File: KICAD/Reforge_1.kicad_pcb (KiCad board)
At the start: 2 copper layers, 57.9 x 76 mm, 94 parts, among them J1 USB_C_Receptacle_USB2.0_16P, J10 Conn_01x14_Pin, J11 Conn_01x12_Pin, J12 Conn_01x12_Pin, J14 Conn_01x12_Pin, J15 Conn_01x12_Pin, J3 Conn_01x02, J8 Conn_01x12_Pin, J9 Conn_01x14_Pin, Q1 SS8050, Q2 SS8050, SW1 SW_Push, SW2 SW_Push, U11 SN74LVC2G125DCUR, U2 CP2102N-Axx-xQFN28, U3 ICE40UP5K-SG48ITR, U4 AP2112K-1.2, U5 ESP32-WROOM-32D, U6 AMS1117-3.3, U8 W25Q32JVSS, Y1 SG-210STF

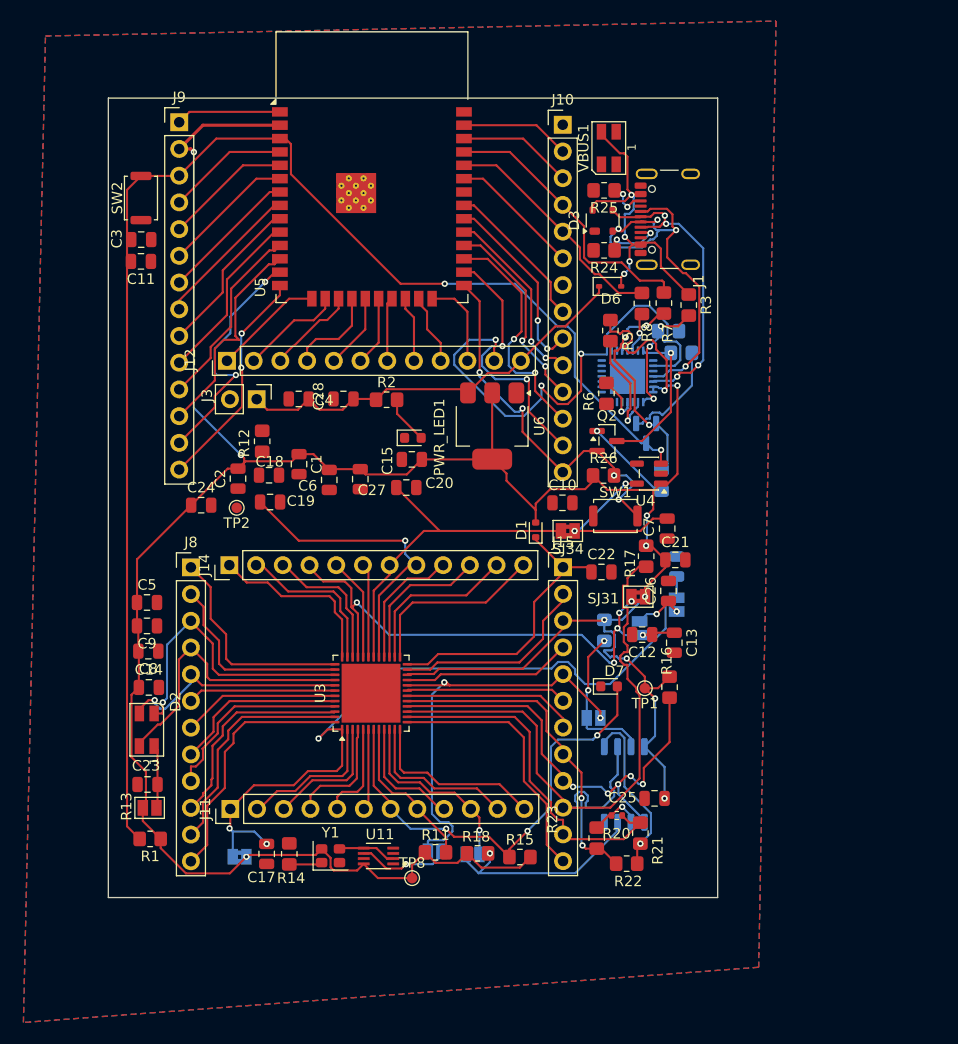
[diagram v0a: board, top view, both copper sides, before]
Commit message: Update schematic and PCB
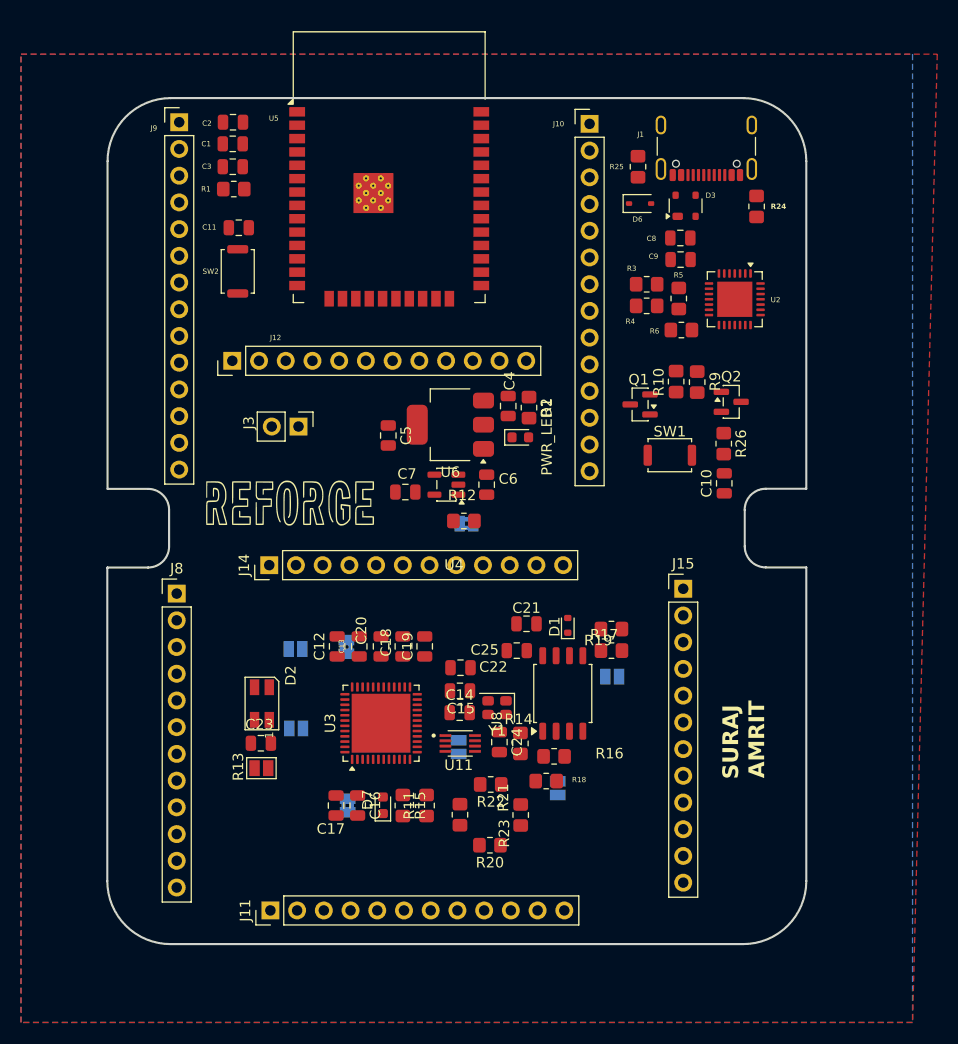
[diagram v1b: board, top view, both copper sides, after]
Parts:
- removed C26, C27, C28: DNI, Capacitor_SMD:C_0805_2012Metric
- removed the G*** at (130.1, 58.2)
- removed R7, R8: 0R(5%), Resistor_SMD:R_0805_2012Metric_Pad1.20x1.40mm_HandSolder
- removed TP1, TP2, TP8: TestPoint, TestPoint:TestPoint_Pad_D1.0mm
- removed VBUS1: TestPoint, LED_SMD:LED_RGB_Wuerth-PLCC4_3.2x2.8mm_150141M173100
- added G***: LOGO, LOGO, F.Cu at (122.5, 87.4)
- added G***: LOGO, LOGO, B.Cu at (129.5, 60.2)
- added G***: LOGO, LOGO, B.Cu at (158.5, 66.4)
- C16, Q1, R10, R19, R4, R9, U2, U8: moved to F.Cu
- R20: footprint Resistor_SMD:R_0402_1005Metric -> Resistor_SMD:R_0805_2012Metric_Pad1.20x1.40mm_HandSolder
- SJ31, SJ34: moved to B.Cu
- moved C8 64.0 mm to (159.4, 60.4), turned to 0 degrees
- moved R1 62.3 mm to (117.0, 55.8)
- moved C9 61.5 mm to (159.4, 62.5), turned to 0 degrees
- moved SJ26 38.0 mm to (122.9, 107.0), turned to 0 degrees
- moved C16 37.9 mm to (128.7, 114.4), turned to -90 degrees
- moved C24 36.2 mm to (142.2, 108.3), turned to -90 degrees
- moved C2 33.9 mm to (116.9, 49.4), turned to 0 degrees
- moved SJ19 32.8 mm to (122.8, 99.5), turned to 0 degrees
- moved C1 31.1 mm to (116.8, 51.5), turned to 180 degrees
- moved C13 30.0 mm to (128.9, 99.2), turned to 90 degrees
- moved C14 29.6 mm to (138.4, 105.5)
- moved C12 29.0 mm to (126.8, 99.2), turned to 90 degrees
- moved SJ31 28.2 mm to (127.7, 99.3), turned to -90 degrees
- moved C5 27.9 mm to (131.6, 79.2), turned to -90 degrees
- moved C7 25.1 mm to (133.3, 84.6), turned to 180 degrees
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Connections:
- J10 pad 4: /TXD0 -> /RXD
- Q2 pad 2: /IO0 -> /~{DTR}
- Q2 pad 3: /~{DTR} -> /IO0
- U2 pad 26: /TXD -> /RXD0
- U5 pad 35: /TXD0 -> /RXD
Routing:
- net /VDD33: track 275.1 -> 0.00 mm, vias 12 -> 0
- net /EN: track 132.6 -> 0.00 mm, vias 2 -> 0
- net /VCCIO_2: track 72.4 -> 0.00 mm, vias 3 -> 0
- net /FT_SCK: track 67.6 -> 0.00 mm
- net /VCCIO_0: track 51.8 -> 0.00 mm, vias 6 -> 0
- net /CLK: track 48.1 -> 0.00 mm, vias 3 -> 0
- net /CDONE: track 43.8 -> 0.00 mm, vias 3 -> 0
- net /FT_SSn: track 43.0 -> 0.00 mm, vias 5 -> 0
- net /+1.2V_CORE: track 42.3 -> 0.00 mm
- net /USB_DP: track 41.2 -> 0.00 mm, vias 4 -> 0
- net /IOB_25B_G3: track 41.1 -> 0.00 mm, vias 2 -> 0
- net /EXT_5V: track 39.4 -> 0.00 mm
- net /IO0: track 36.2 -> 0.00 mm, vias 4 -> 0
- net /FPGA_SO: track 33.8 -> 0.00 mm
- net /FPGA_SI: track 31.8 -> 0.00 mm, vias 2 -> 0
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- added copper zone on F.Cu, net /VDD33
- removed copper zone on F.Cu, net GND
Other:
- board size 57.9 x 76 mm -> 66.5 x 80.4 mm
- board text added: "AMRIT"
- board text added: "SURAJ"
